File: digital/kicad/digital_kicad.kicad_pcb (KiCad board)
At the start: 2 copper layers, 100 x 100 mm, 17 parts, among them J1 Barrel_Jack_Switch, J2 Screw_Terminal_01x02, Q1 2N3904, Q2 2N3904, Q4 2N3904, SW1 SW_SPST

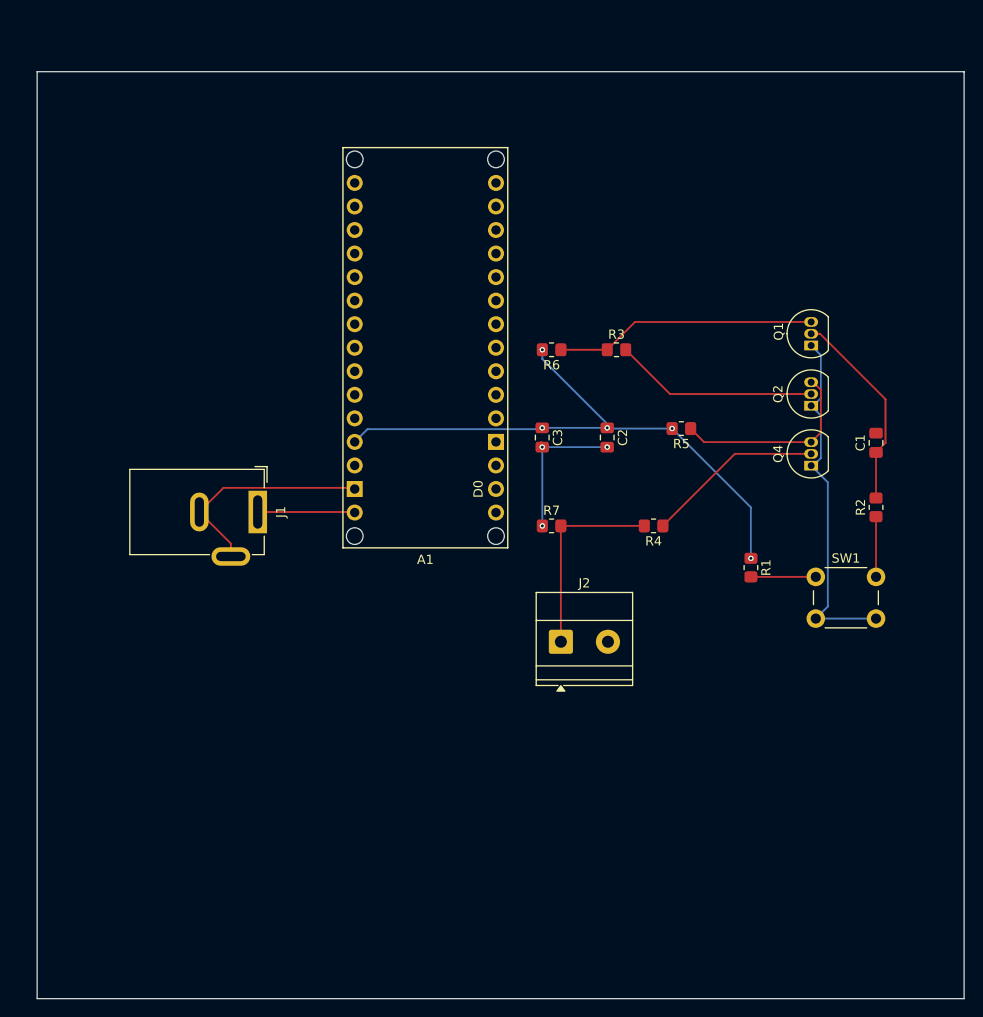
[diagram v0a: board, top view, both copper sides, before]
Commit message: updated pcb with Jarek's changes
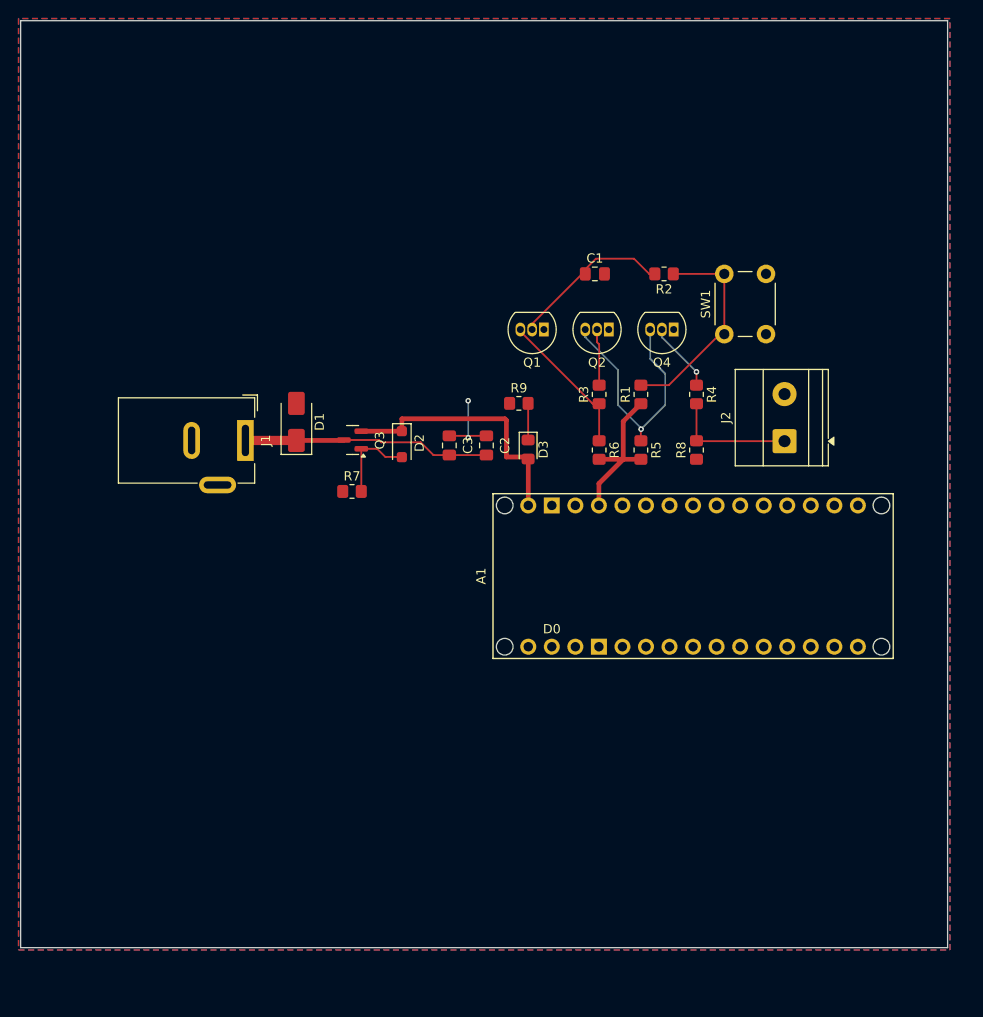
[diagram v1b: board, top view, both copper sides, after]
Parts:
- added D1: SMAJ13A, Diode_SMD:D_SMA, F.Cu at (128.0, 66.8)
- added D2: BZT52Bxx, Diode_SMD:D_SOD-123F, F.Cu at (139.3, 69.2)
- added D3: LED, LED_SMD:LED_0805_2012Metric_Pad1.15x1.40mm_HandSolder, F.Cu at (153.0, 69.8)
- added Q3: FDN340P, Package_TO_SOT_SMD:SOT-23, F.Cu at (134.0, 68.7)
- added R8: 33k, Resistor_SMD:R_0805_2012Metric_Pad1.20x1.40mm_HandSolder, F.Cu at (171.1, 69.8)
- added R9: 1k, Resistor_SMD:R_0805_2012Metric_Pad1.20x1.40mm_HandSolder, F.Cu at (152.0, 64.8)
- J1: footprint Connector_BarrelJack:BarrelJack_GCT_DCJ200-10-A_Horizontal -> Connector_BarrelJack:BarrelJack_Wuerth_6941xx301002
- R7: value 33k -> 100k
- moved A1 68.4 mm to (192.4, 83.4), turned to 90 degrees
- moved C1 35.4 mm to (160.2, 50.8), turned to 0 degrees
- moved R2 34.0 mm to (167.6, 50.8), turned to 180 degrees
- moved J2 32.4 mm to (180.6, 68.9), turned to 90 degrees
- moved Q1 28.9 mm to (154.7, 56.8), turned to 180 degrees
- moved SW1 28.0 mm to (174.1, 57.3), turned to 90 degrees
- moved Q2 23.3 mm to (161.7, 56.8), turned to 180 degrees
- moved R1 22.1 mm to (165.1, 63.8), turned to 90 degrees
- moved R7 21.9 mm to (134.0, 74.3)
- moved Q4 20.9 mm to (168.7, 56.8), turned to 180 degrees
- moved R4 14.9 mm to (171.1, 63.8), turned to -90 degrees
- moved C2 13.1 mm to (148.5, 69.3), turned to 90 degrees
- moved R6 12.0 mm to (160.6, 69.8), turned to -90 degrees
- moved C3 10.1 mm to (144.5, 69.3), turned to 90 degrees
- moved J1 7.83 mm to (122.5, 68.8)
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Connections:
- net Net-(Q2-C) renamed /OUT
- net SW renamed /SW
- net inv. SW renamed /inv. SW
- C2 pad 1: +5V -> Net-(D1-A1)
- C3 pad 1: +5V -> Net-(D1-A1)
- J1 pad 1: /VDC -> Net-(D1-A1)
- J2 pad 1: Net-(J2-Pin_1) -> /DIG_IN
- R4 pad 2: Net-(J2-Pin_1) -> /DIG_IN
- R7 pad 2: Net-(J2-Pin_1) -> Net-(D2-A)
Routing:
- net GND: track 79.2 -> 8.18 mm, vias 6 -> 2
- net +5V: track 65.1 -> 17.4 mm, vias 6 -> 0
- net Net-(D1-A1): track 0.00 -> 26.7 mm
- net Net-(J2-Pin_1): track 21.5 -> 0.00 mm
- net /VDC: track 10.5 -> 28.6 mm
- net Net-(Q2-B): track 22.0 -> 6.10 mm
- net /DIG_IN: track 0.00 -> 13.5 mm
- net /inv. SW: track 28.2 -> 15.9 mm
- net A: track 19.2 -> 7.57 mm, vias 0 -> 1
- net /SW: track 13.5 -> 23.3 mm
- net Net-(D2-A): track 0.00 -> 9.35 mm
- net /OUT: track 21.1 -> 27.1 mm, vias 0 -> 1
- net Net-(Q1-B): track 22.0 -> 17.7 mm
- net Net-(D3-K): track 0.00 -> 3.95 mm
- added copper zone on B.Cu, net GND
- added copper zone on F.Cu, net GND
